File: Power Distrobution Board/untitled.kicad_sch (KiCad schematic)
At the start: 11 parts, among them J3 AT15-4P-BM01, K2 EW60-1A3-CL12D04,00000, K3 AZ2150-1A-12DEF

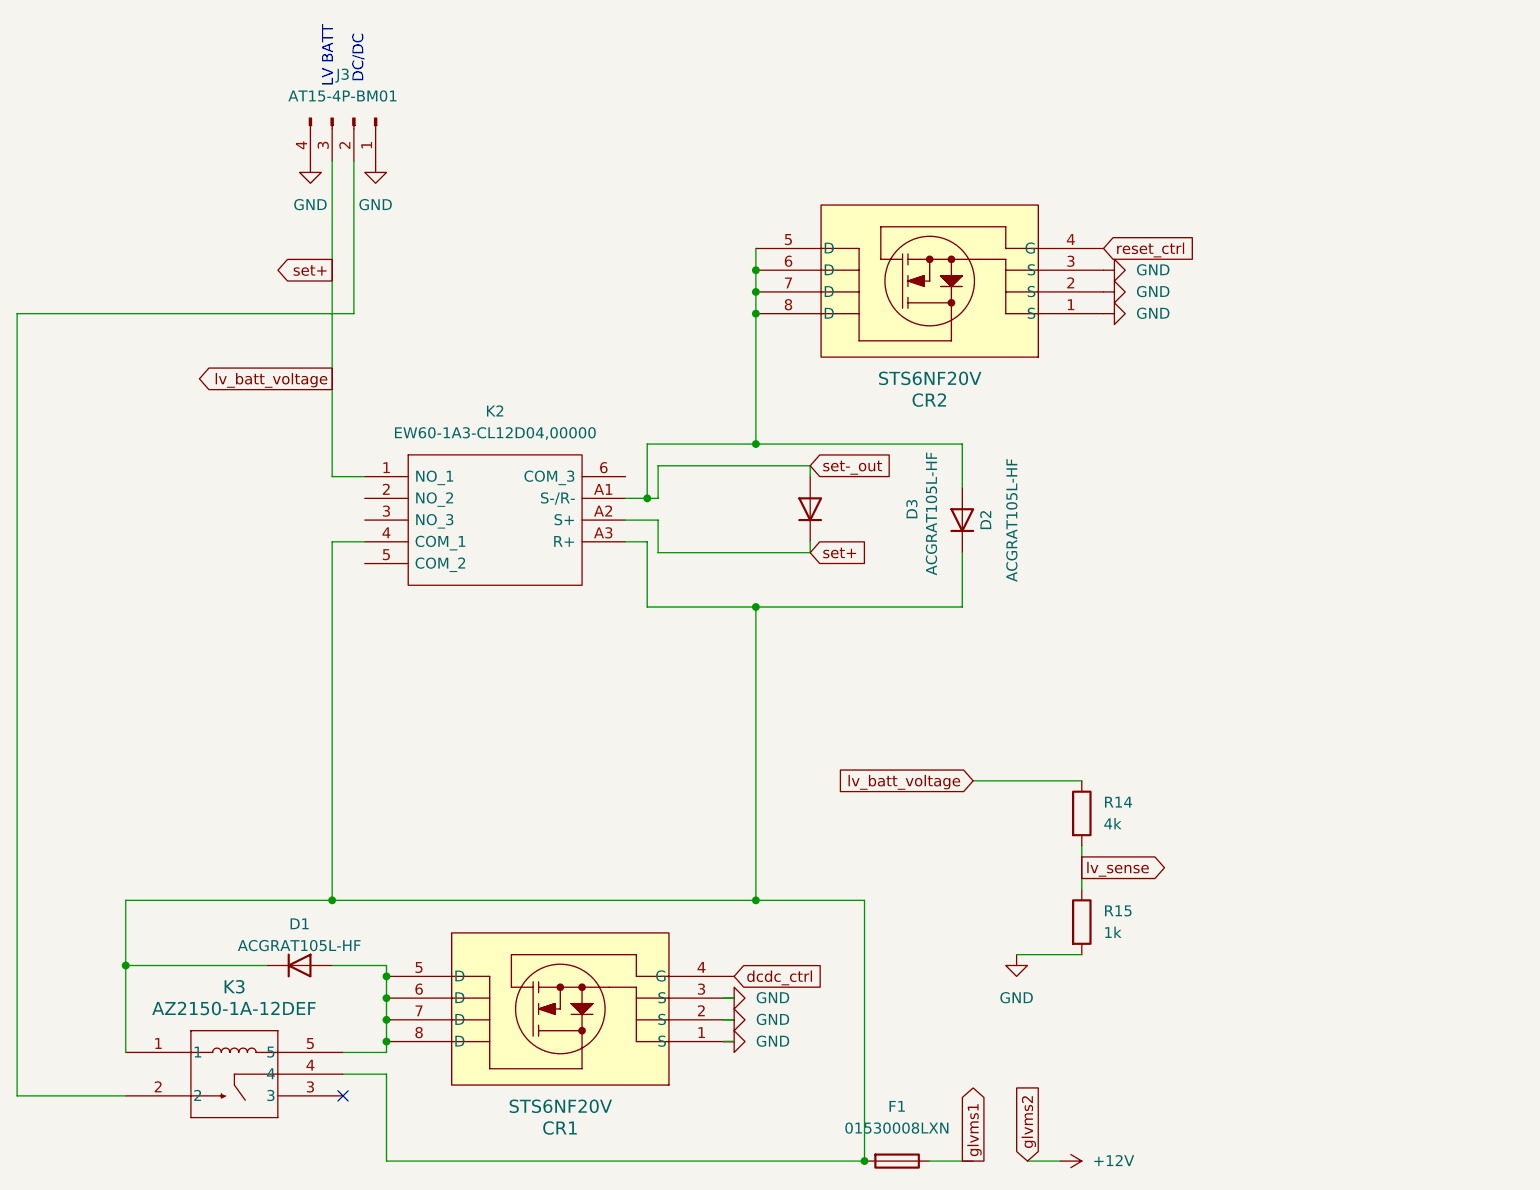
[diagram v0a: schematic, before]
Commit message: v2.2
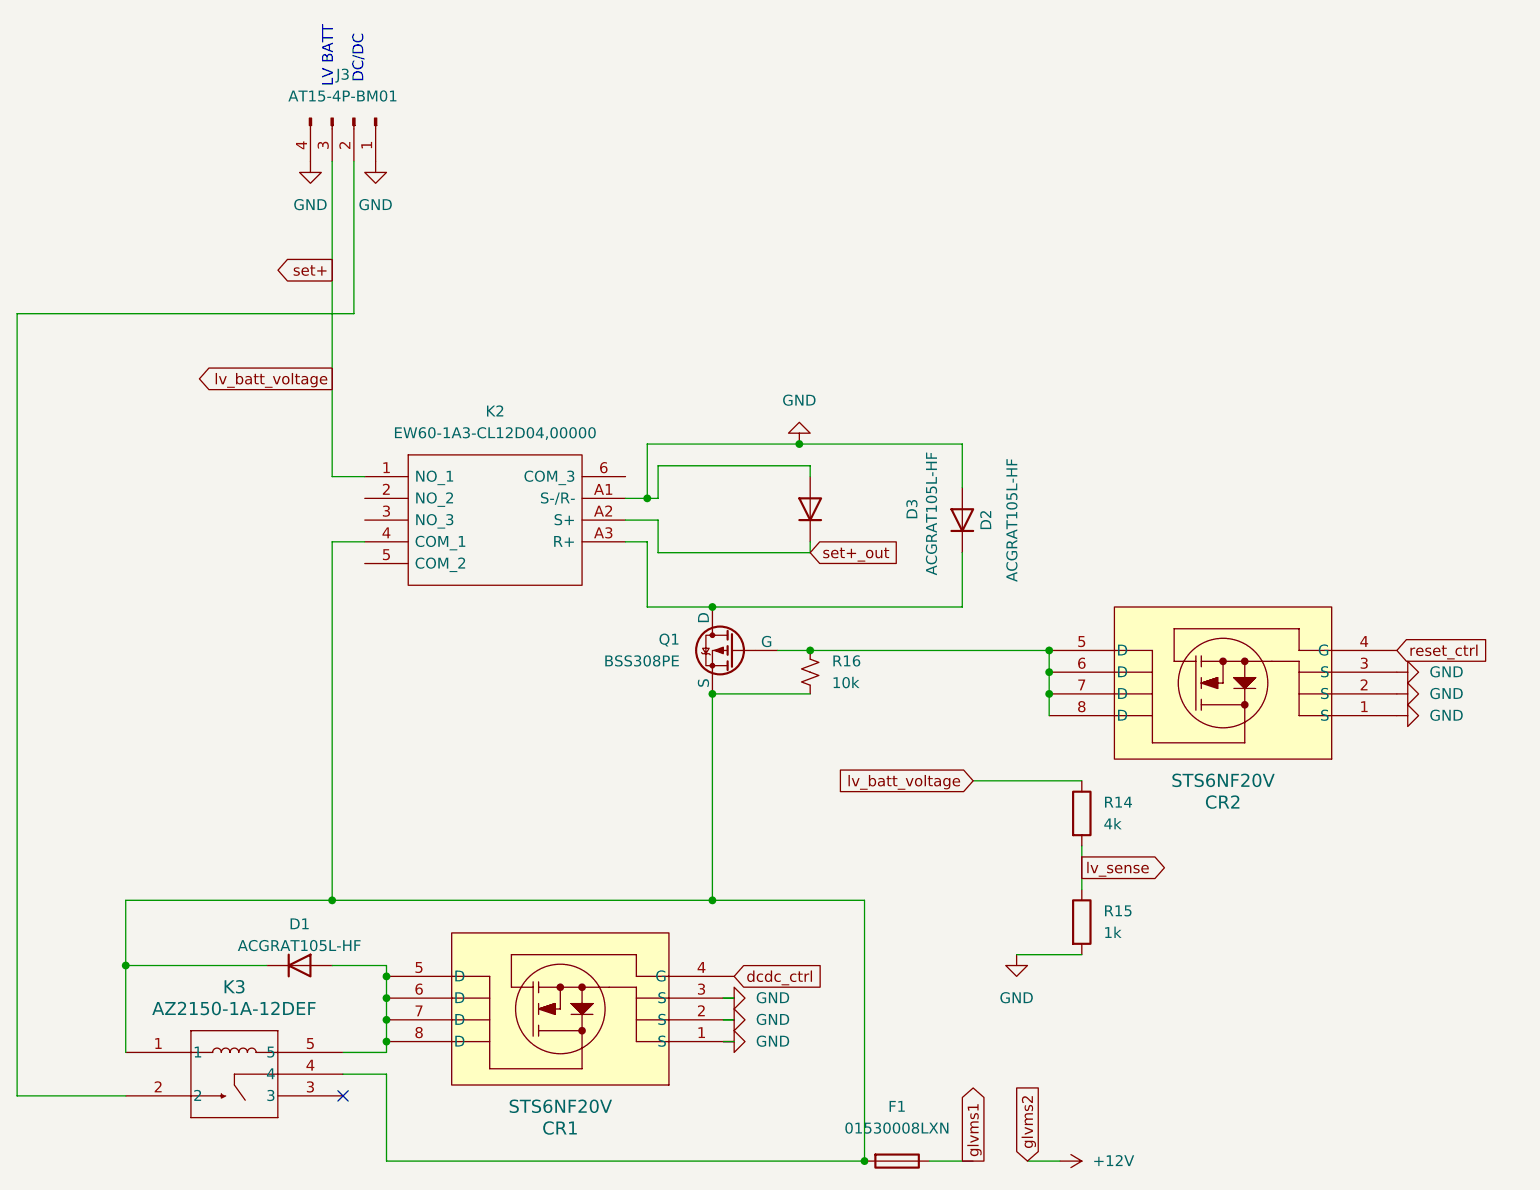
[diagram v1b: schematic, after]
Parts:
- added Q1: BSS308PE, Package_TO_SOT_SMD:SOT-23_Handsoldering, symbol FS_3_Global_Symbol_Library:BSS308PE
- added R16: 10k, Resistor_SMD:R_0805_2012Metric_Pad1.20x1.40mm_HandSolder, symbol Device:R_Small_US
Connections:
- net GND: now also D2.2 (A), D3.2 (A), K2.A1 (S-/R-)
- net lv_batt_voltage: no longer D3.1 (K), K2.A2 (S+)
- net at D1.1 (K), F1.2, K2.4 (COM_1)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: now also Q1.2 (S), R16.1; no longer D2.1 (K), K2.A3 (R+)
- net set-_out: no longer names the net of CR2.5 (D), CR2.6 (D), CR2.7 (D), CR2.8 (D)
- net set-_out: now also Q1.1 (G), R16.2; no longer D2.2 (A), D3.2 (A), K2.A1 (S-/R-)
- new net: D2.1 (K), K2.A3 (R+), Q1.3 (D)
- new net set+_out: D3.1 (K), K2.A2 (S+)
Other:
- moved on the sheet: CR2
